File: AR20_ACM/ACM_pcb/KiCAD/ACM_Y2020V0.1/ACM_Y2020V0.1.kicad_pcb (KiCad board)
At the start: 2 copper layers, 26.5 x 26.6 mm, 21 parts, among them J1 TC2030-MCP-NL, J2 Conn_02x15_Odd_Even, U1 ATmega328PB-AU, U2 MCP25625-x-SS, U3 SPX3819M5-L-5-0, Y1 16.0Mhz

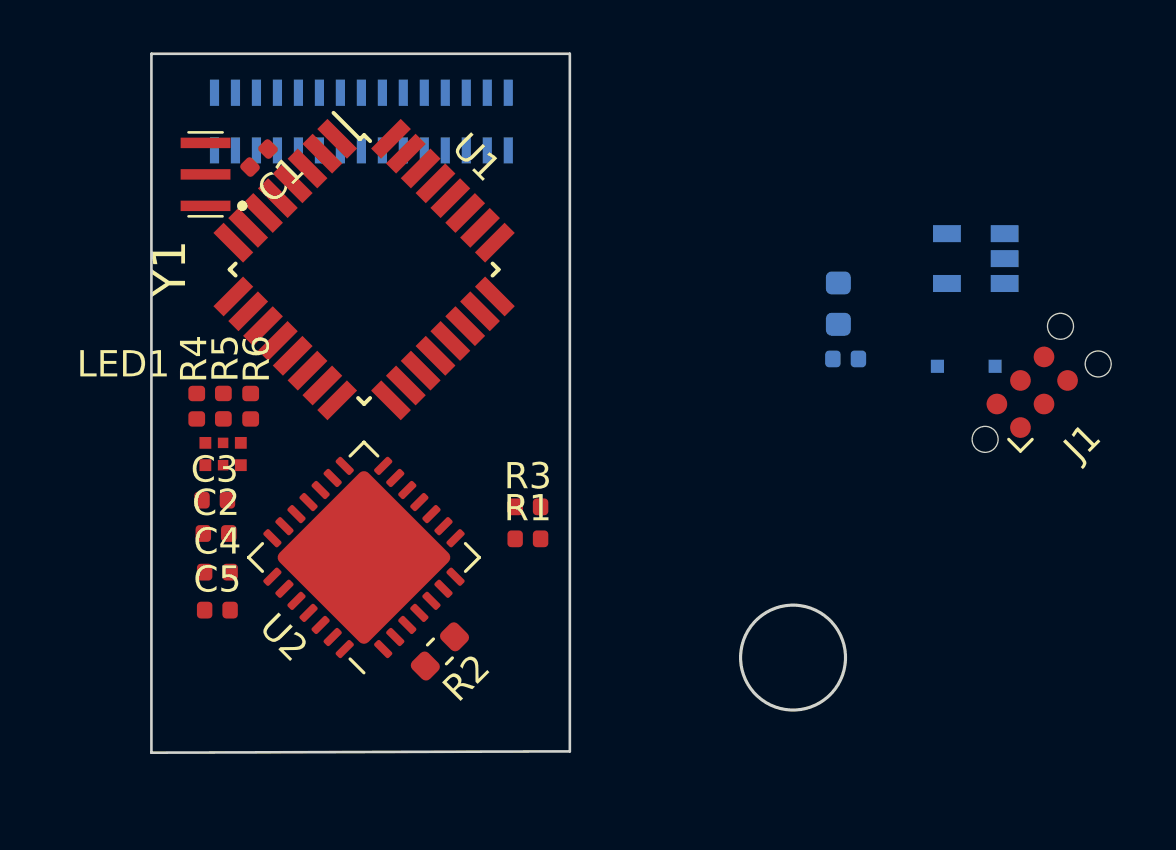
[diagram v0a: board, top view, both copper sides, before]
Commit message: Changelog for 28.07.2019
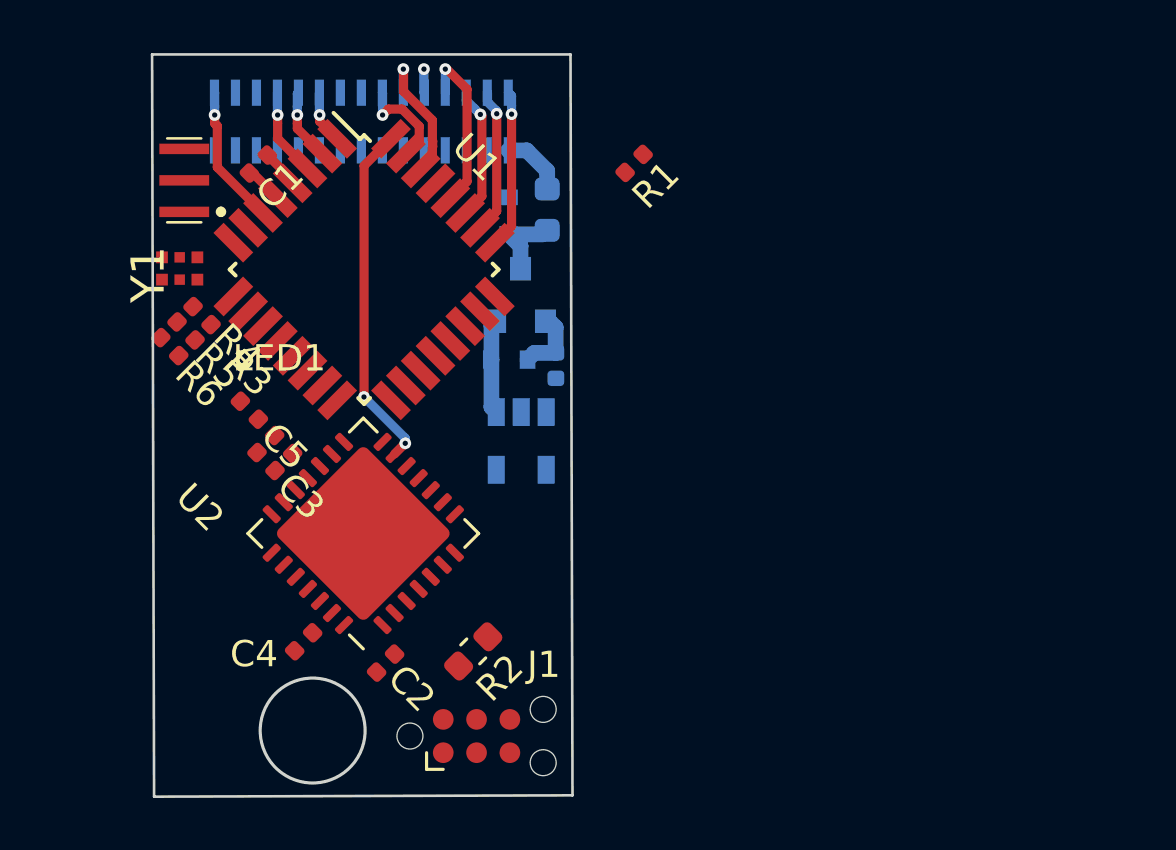
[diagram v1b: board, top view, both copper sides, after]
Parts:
- added Q1: Q_PMOS_DGS, Package_TO_SOT_SMD:SOT-23, B.Cu at (146.7, 86.4)
- added R7: 100K Ohm, Resistor_SMD:R_0402_1005Metric, B.Cu at (148.1, 89.1)
- D1: footprint Diode_SMD:D_SOD-323F -> Diode_SMD:D_SOD-523
- D2: value D_Small -> 2.4V; footprint Diode_SMD:D_0402_1005Metric -> Diode_SMD:D_SOD-523
- F1: value 200mA -> 250mA
- moved J1 24.9 mm to (145.0, 103.2), turned to 0 degrees
- moved U3 18.7 mm to (146.7, 92.0), turned to 270 degrees
- moved D1 18.4 mm to (146.3, 83.4), turned to 90 degrees
- moved R1 14.9 mm to (151.0, 81.4), turned to 225 degrees
- moved D2 12.8 mm to (146.3, 88.9)
- moved F1 11.7 mm to (147.7, 83.2)
- moved R3 9.61 mm to (137.7, 92.1), turned to 135 degrees
- moved C2 8.14 mm to (141.6, 100.4), turned to 225 degrees
- moved C5 7.72 mm to (136.4, 90.8), turned to 135 degrees
- moved LED1 6.23 mm to (134.4, 85.8), turned to 180 degrees
- moved C4 4.23 mm to (138.4, 99.6), turned to 45 degrees
- moved R6 3.83 mm to (133.3, 88.4), turned to 315 degrees
- moved R4 3.46 mm to (134.6, 87.2), turned to 315 degrees
- moved R5 3.20 mm to (134.0, 87.8), turned to 315 degrees
- moved C3 2.45 mm to (137.0, 92.8), turned to 135 degrees
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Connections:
- net /U-Pin28 renamed Net-(J2-Pad28)
- net Net-(J2-Pad13) renamed /U-Pin13
- net Net-(J2-Pad15) renamed /U-Pin15
- net Net-(J2-Pad17) renamed /U-Pin17
- net Net-(J2-Pad19) renamed /U-Pin19
- net Net-(J2-Pad21) renamed /U-Pin21
- net Net-(J2-Pad25) renamed /U-Pin25
- D1 pad 1: +12V -> Net-(D1-Pad1)
- D2 pad 2: GND -> Net-(D2-Pad2)
- F1 pad 1: Net-(D2-Pad1) -> Net-(D1-Pad1)
- J2 pad 11: Net-(J2-Pad11) -> /U-Pin11
- J2 pad 16: /U-Pin16 -> GND
- J2 pad 18: /U-Pin18 -> GND
- J2 pad 2: GND -> /U-Pin2
- J2 pad 23: Net-(J2-Pad23) -> /U-Pin23
- J2 pad 26: /U-Pin26 -> Net-(J2-Pad26)
- J2 pad 27: Net-(J2-Pad27) -> /U-Pin27
- J2 pad 29: Net-(J2-Pad29) -> /U-Pin29
- J2 pad 30: Net-(J2-Pad30) -> /U-Pin30
- J2 pad 4: GND -> /U-Pin4
- J2 pad 5: +5V -> /U-Pin5
- J2 pad 6: GND -> /U-Pin6
- J2 pad 7: Net-(J2-Pad7) -> /U-Pin7
- J2 pad 9: Net-(J2-Pad9) -> /U-Pin9
- R2 pad 1: /CANH -> /U-Pin27
- R2 pad 2: /CANL -> /U-Pin29
- U1 pad 1: Net-(U1-Pad1) -> /U-Pin20
- U1 pad 10: Net-(U1-Pad10) -> /U-Pin23
- U1 pad 19: /U-Pin8 -> /U-Pin11
- U1 pad 2: Net-(U1-Pad2) -> /U-Pin22
- U1 pad 22: /U-Pin10 -> /U-Pin9
- U1 pad 23: /U-Pin12 -> /U-Pin7
- U1 pad 24: /U-Pin14 -> /U-Pin5
- U1 pad 25: /U-Pin16 -> /U-Pin2
- U1 pad 26: /U-Pin18 -> /U-Pin4
- U1 pad 27: /U-Pin20 -> /U-Pin6
- U1 pad 28: /U-Pin22 -> /U-Pin8
- U1 pad 3: Net-(U1-Pad3) -> /U-Pin24
- U1 pad 30: /U-Pin24 -> /U-Pin12
- U1 pad 31: /U-Pin26 -> /U-Pin14
- U1 pad 6: Net-(U1-Pad6) -> /U-Pin30
- U2 pad 3: /CANL -> /U-Pin29
- U2 pad 4: /CANH -> /U-Pin27
- U2 pad 5: Net-(U2-Pad5) -> GND
- U2 pad 9: Net-(U2-Pad9) -> /CLK_MCP
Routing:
- net /CAN_INT: track 0.00 -> 13.3 mm, vias 0 -> 2
- net /U-Pin8: track 0.00 -> 6.46 mm, vias 0 -> 1
- net /U-Pin2: track 0.00 -> 6.03 mm, vias 0 -> 1
- net /U-Pin4: track 0.00 -> 5.56 mm, vias 0 -> 1
- net /U-Pin30: track 0.00 -> 5.35 mm, vias 0 -> 1
- net /U-Pin12: track 0.00 -> 5.34 mm, vias 0 -> 1
- net /U-Pin6: track 0.00 -> 5.10 mm, vias 0 -> 1
- net /U-Pin14: track 0.00 -> 3.87 mm, vias 0 -> 1
- net Net-(D2-Pad1): track 0.00 -> 3.62 mm
- net /U-Pin24: track 0.00 -> 3.37 mm, vias 0 -> 1
- net Net-(D1-Pad1): track 0.00 -> 3.05 mm
- net /U-Pin22: track 0.00 -> 2.74 mm, vias 0 -> 1
- net Net-(D2-Pad2): track 0.00 -> 2.64 mm
- net +12V: track 0.00 -> 2.50 mm
- net /U-Pin20: track 0.00 -> 2.04 mm, vias 0 -> 1
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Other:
- board size 26.5 x 26.6 mm -> 16 x 28.3 mm
- net class Default: clearance 0.2 -> 0.0889; trace_width 0.25 -> 0.0889; via_dia 0.8 -> 0.45; via_drill 0.4 -> 0.2
- rule trace_clearance: 0.2 -> 0.0889
- rule trace_min: 0.2 -> 0.0889
- rule via_min_drill: 0.3 -> 0.2
- rule via_min_size: 0.2 -> 0.45

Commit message: Changelog for 29.07.2019
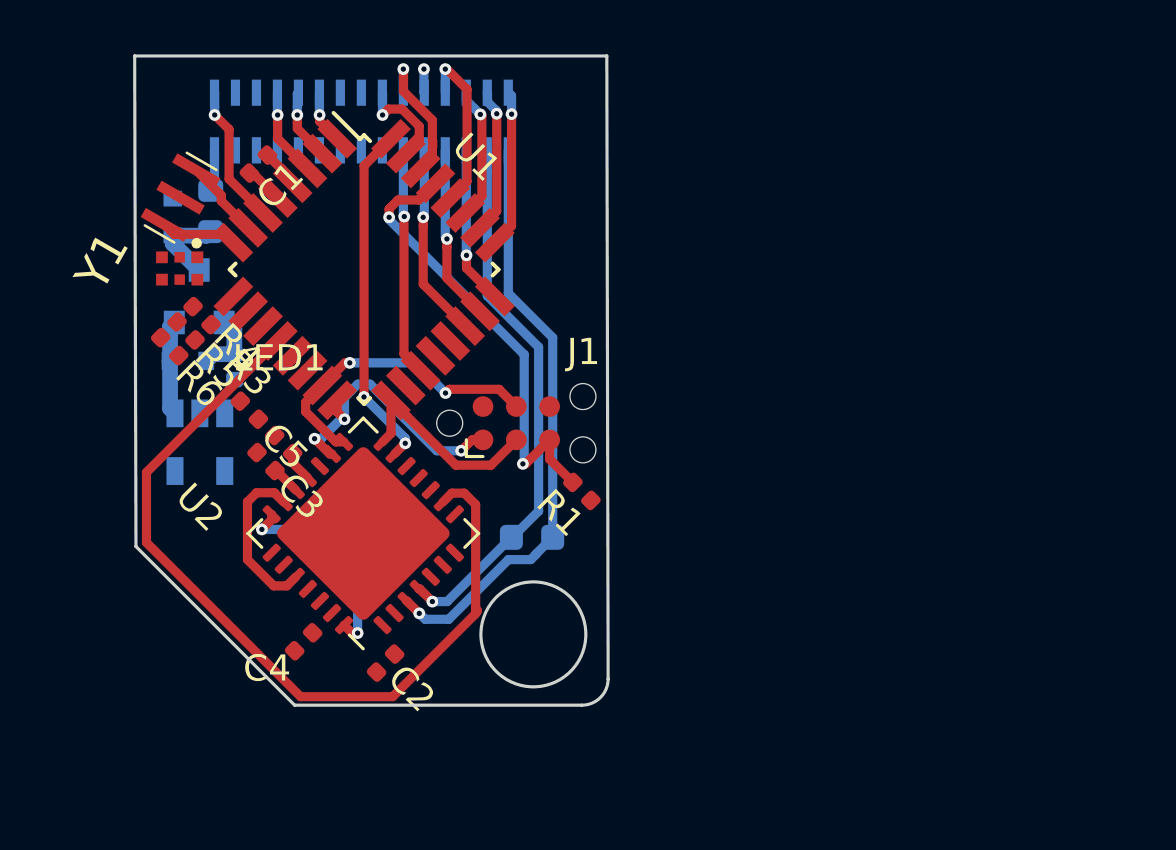
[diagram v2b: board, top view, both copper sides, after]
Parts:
- R2: moved to B.Cu
- moved F1 12.8 mm to (134.9, 83.2)
- moved D1 12.8 mm to (133.4, 83.4)
- moved R1 12.7 mm to (149.1, 93.9), turned to 135 degrees
- moved D2 12.3 mm to (134.0, 88.9)
- moved Q1 12.3 mm to (134.5, 86.5)
- moved R7 12.3 mm to (135.8, 89.2)
- moved U3 12.3 mm to (134.5, 92.0)
- moved J1 12.0 mm to (146.6, 91.3)
- moved R2 4.89 mm to (147.2, 95.7), turned to 0 degrees
- moved Y1 0.89 mm to (134.1, 82.9), turned to 60 degrees
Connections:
- net /U-Pin10 renamed Net-(J2-Pad10)
- net /U-Pin25 renamed Net-(J2-Pad25)
- J2 pad 1: +12V -> /U-Pin1
- J2 pad 27: /U-Pin27 -> +5V
- J2 pad 29: /U-Pin29 -> +12V
- J2 pad 3: +5V -> /U-Pin3
- R2 pad 1: /U-Pin27 -> /U-Pin3
- R2 pad 2: /U-Pin29 -> /U-Pin1
- U2 pad 3: /U-Pin29 -> /U-Pin1
- U2 pad 4: /U-Pin27 -> /U-Pin3
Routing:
- net /CLK_MCP: track 0.00 -> 31.8 mm
- net /U-Pin1: track 0.00 -> 22.6 mm, vias 0 -> 1
- net /U-Pin3: track 0.00 -> 20.8 mm, vias 0 -> 1
- net /Reset: track 0.00 -> 17.4 mm, vias 0 -> 2
- net /MOSI: track 0.00 -> 11.8 mm, vias 0 -> 2
- net /MISO: track 0.00 -> 10.7 mm, vias 0 -> 3
- net /U-Pin11: track 0.00 -> 8.68 mm, vias 0 -> 1
- net /SCK: track 0.00 -> 7.92 mm
- net /U-Pin9: track 0.00 -> 7.38 mm, vias 0 -> 1
- net Net-(U2-Pad21): track 0.00 -> 7.34 mm, vias 0 -> 2
- net /U-Pin7: track 0.00 -> 6.68 mm, vias 0 -> 1
- net Net-(U2-Pad20): track 0.00 -> 6.28 mm
- net /U-Pin5: track 0.00 -> 6.02 mm, vias 0 -> 1
- net Net-(U1-Pad7): track 0.00 -> 3.01 mm
- net Net-(U1-Pad8): track 0.00 -> 2.89 mm
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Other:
- board size 16 x 28.3 mm -> 18.1 x 24.8 mm
